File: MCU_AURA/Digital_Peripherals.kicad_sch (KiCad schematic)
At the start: 28 parts, among them IC1 PCA9685PW,118, IC2 W25Q128JVSIQ, J1 TF-CARD_H1.8, Q300 BSS138, Q301 BSS138, Q302 BSS138, U300 ICM-20948, U301 BMP280

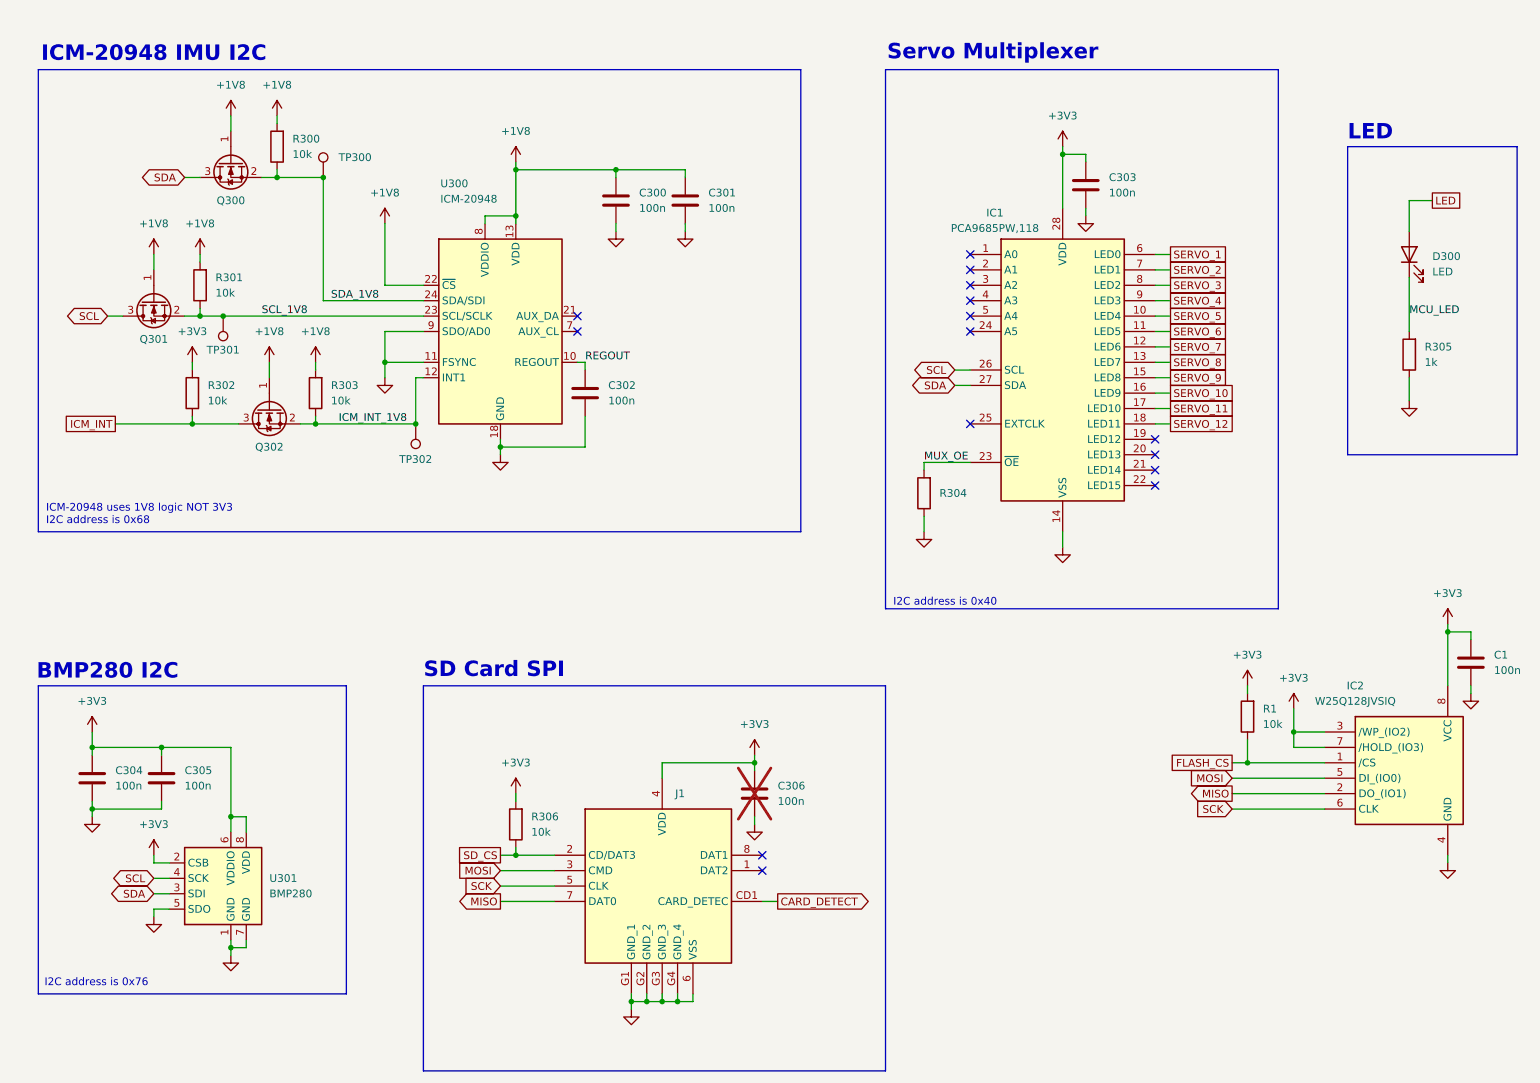
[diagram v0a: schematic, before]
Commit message: Second Iteration MCU
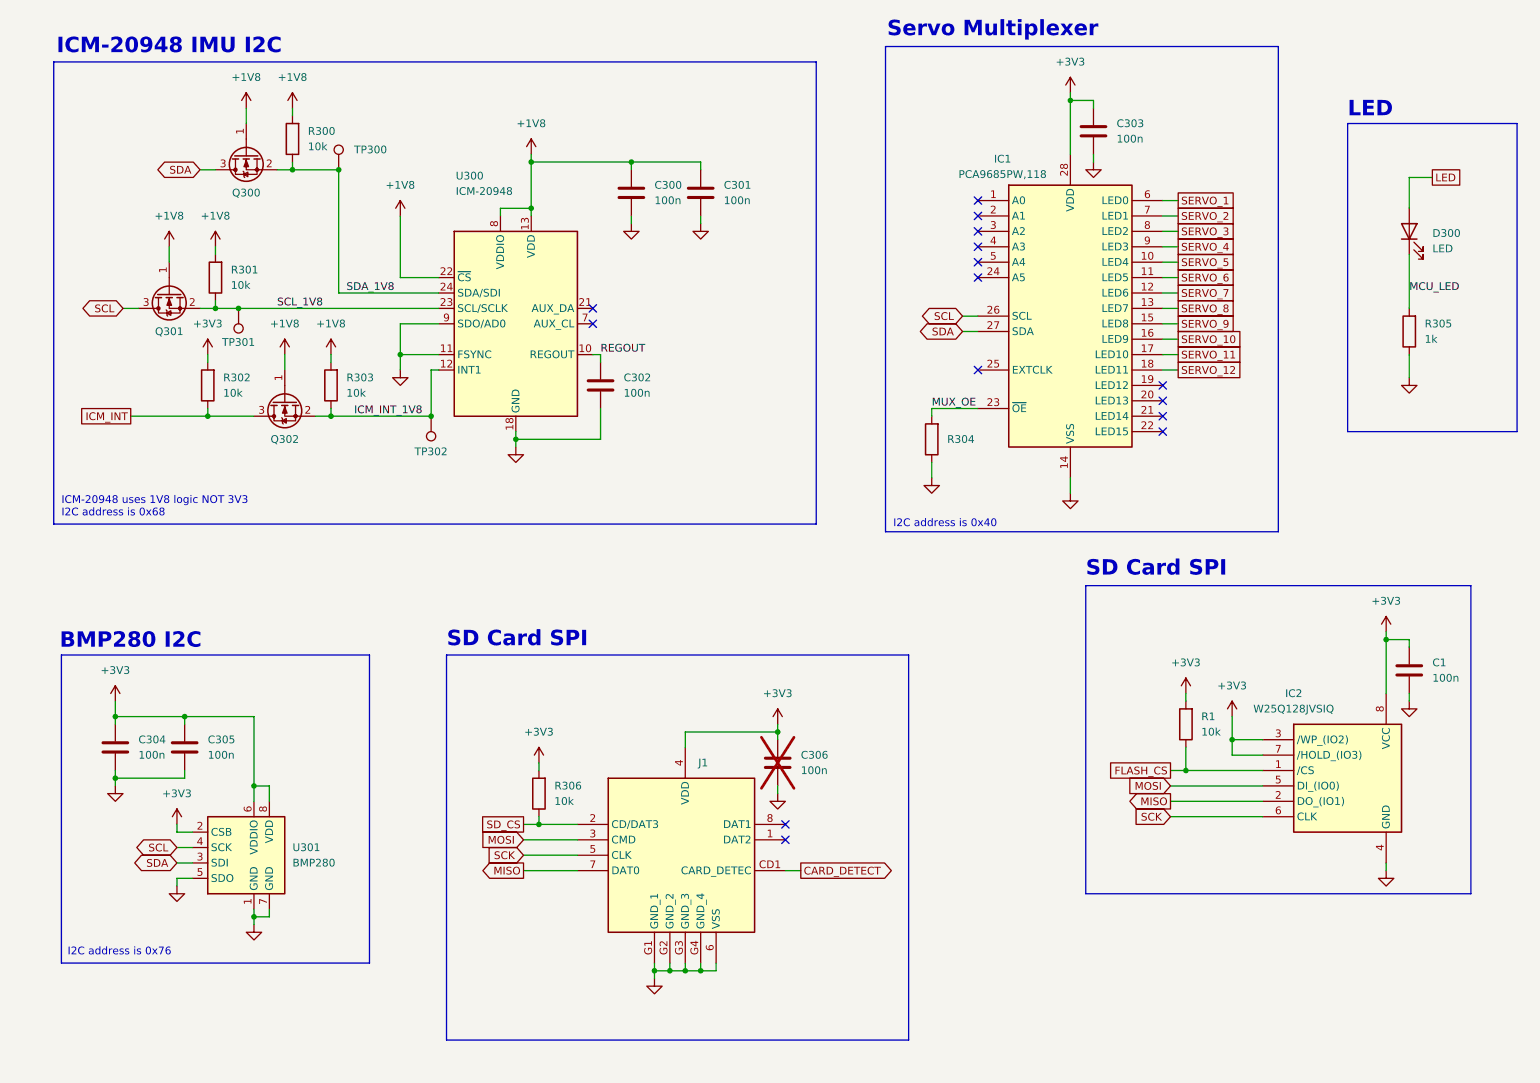
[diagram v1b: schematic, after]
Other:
- moved on the sheet: C1, C300, C301, C302, C303, C304, C305, C306, D300, IC1, IC2, J1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
